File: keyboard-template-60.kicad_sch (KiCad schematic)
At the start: 168 parts, among them J1 USB_C_Receptacle_USB2.0, J2 Conn_01x04_MountingPin, SW1 SW_Reset, U1 ATmega32U4-M, U2 SRV05-4, Y1 16MHz

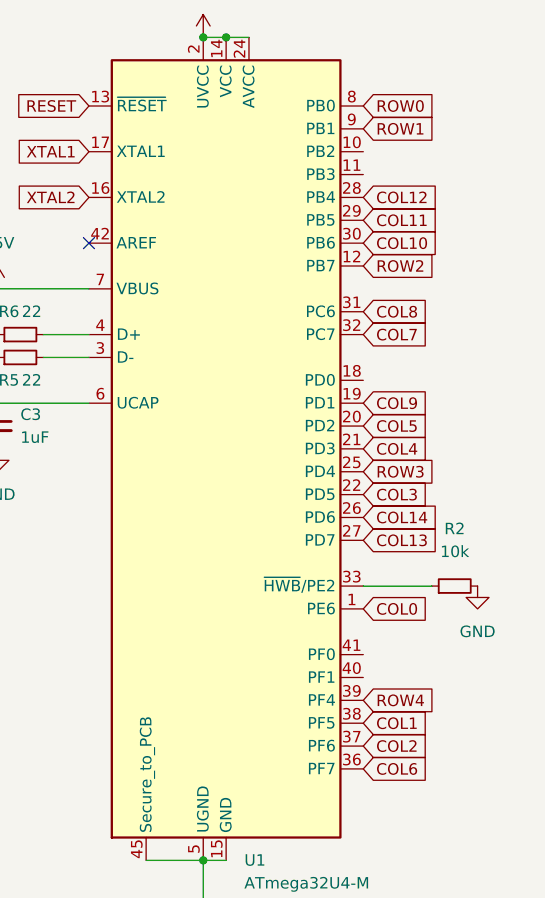
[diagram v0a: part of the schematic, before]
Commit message: Update schematics and BOM
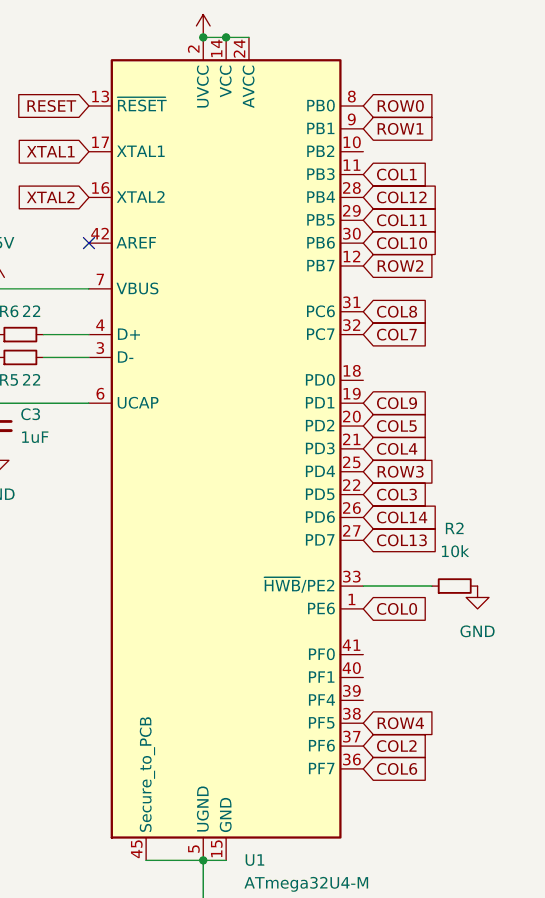
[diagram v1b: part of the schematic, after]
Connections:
- net COL1: now also U1.11 (PB3); no longer U1.38 (PF5)
- net ROW4: now also U1.38 (PF5); no longer U1.39 (PF4)
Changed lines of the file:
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@@
     )
   )
-  (global_label "ROW4" (shape input) (at 370.84 109.22 0) (fields_autoplaced)
+  (global_label "ROW4" (shape input) (at 370.84 111.76 0) (fields_autoplaced)
     (effects (font (size 1.27 1.27)) (justify left))
-    (property "Intersheet References" "${INTERSHEET_REFS}" (id 0) (at 378.5145 109.2994 0)
+    (property "Intersheet References" "${INTERSHEET_REFS}" (id 0) (at 378.5145 111.8394 0)
       (effects (font (size 1.27 1.27)) (justify left) hide)
     )
@@
     )
   )
-  (global_label "COL1" (shape input) (at 370.84 111.76 0) (fields_autoplaced)
+  (global_label "COL1" (shape input) (at 370.84 50.8 0) (fields_autoplaced)
     (effects (font (size 1.27 1.27)) (justify left))
-    (property "Intersheet References" "${INTERSHEET_REFS}" (id 0) (at 378.0912 111.8394 0)
+    (property "Intersheet References" "${INTERSHEET_REFS}" (id 0) (at 378.0912 50.8794 0)
       (effects (font (size 1.27 1.27)) (justify left) hide)
     )

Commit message: Final layout for prototype
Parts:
- Y1: footprint Crystal:Crystal_SMD_3225-4Pin_3.2x2.5mm_HandSoldering -> Crystal:Crystal_SMD_3225-4Pin_3.2x2.5mm
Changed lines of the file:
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@@
     (property "Reference" "Y1" (id 0) (at 298.45 78.74 90))
     (property "Value" "16MHz" (id 1) (at 298.45 81.28 90))
-    (property "Footprint" "Crystal:Crystal_SMD_3225-4Pin_3.2x2.5mm_HandSoldering" (id 2) (at 292.1 81.28 0)
+    (property "Footprint" "Crystal:Crystal_SMD_3225-4Pin_3.2x2.5mm" (id 2) (at 292.1 81.28 0)
       (effects (font (size 1.27 1.27)) hide)
     )
@@
     )
     (path "/40a982a0-a582-4b57-8a47-74dcce3e7b3f"
-      (reference "Y1") (unit 1) (value "16MHz") (footprint "Crystal:Crystal_SMD_3225-4Pin_3.2x2.5mm_HandSoldering")
-    )
-  )
+      (reference "Y1") (unit 1) (value "16MHz") (footprint "Crystal:Crystal_SMD_3225-4Pin_3.2x2.5mm")
+    )
+  )
